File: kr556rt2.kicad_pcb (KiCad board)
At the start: 2 copper layers, 24.8 x 40.1 mm, 2 parts, among them U1 27C512, U2 КР556РТ2

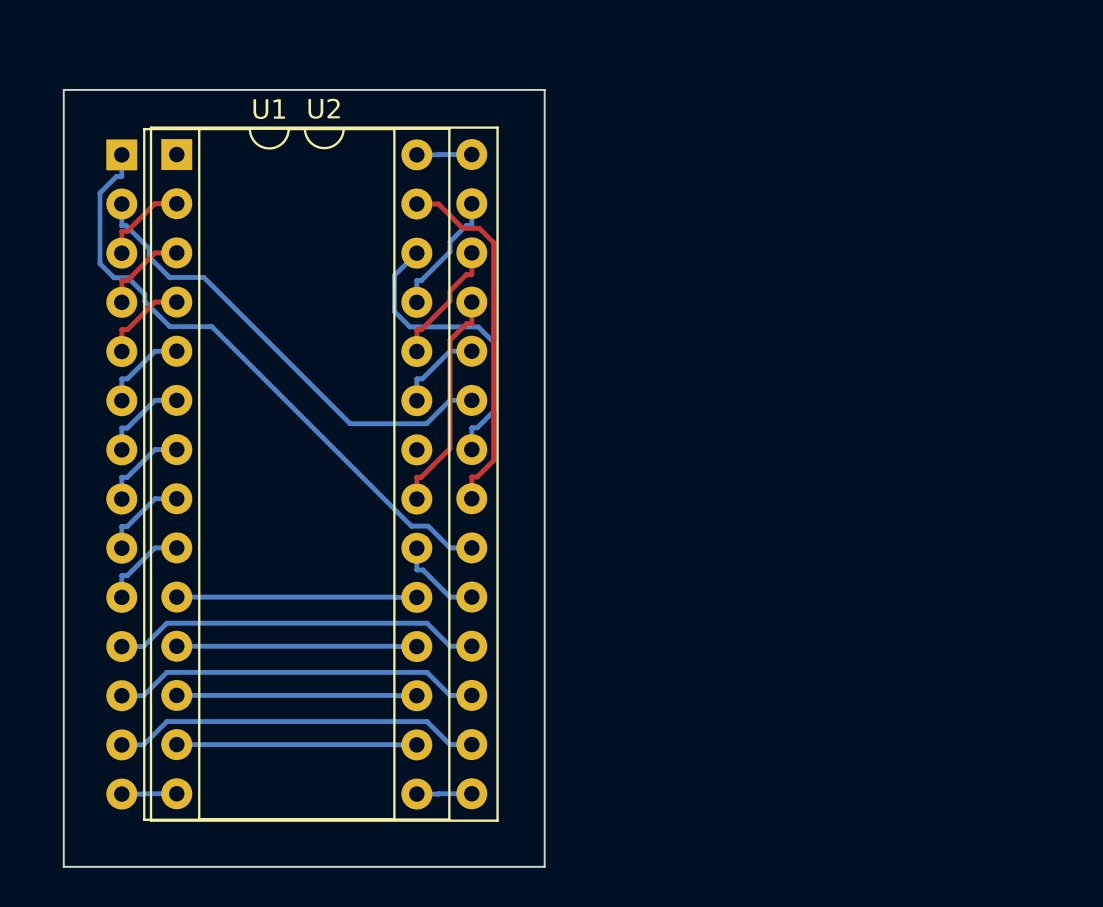
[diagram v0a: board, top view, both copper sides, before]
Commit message: Update kr556rt2.kicad_pcb
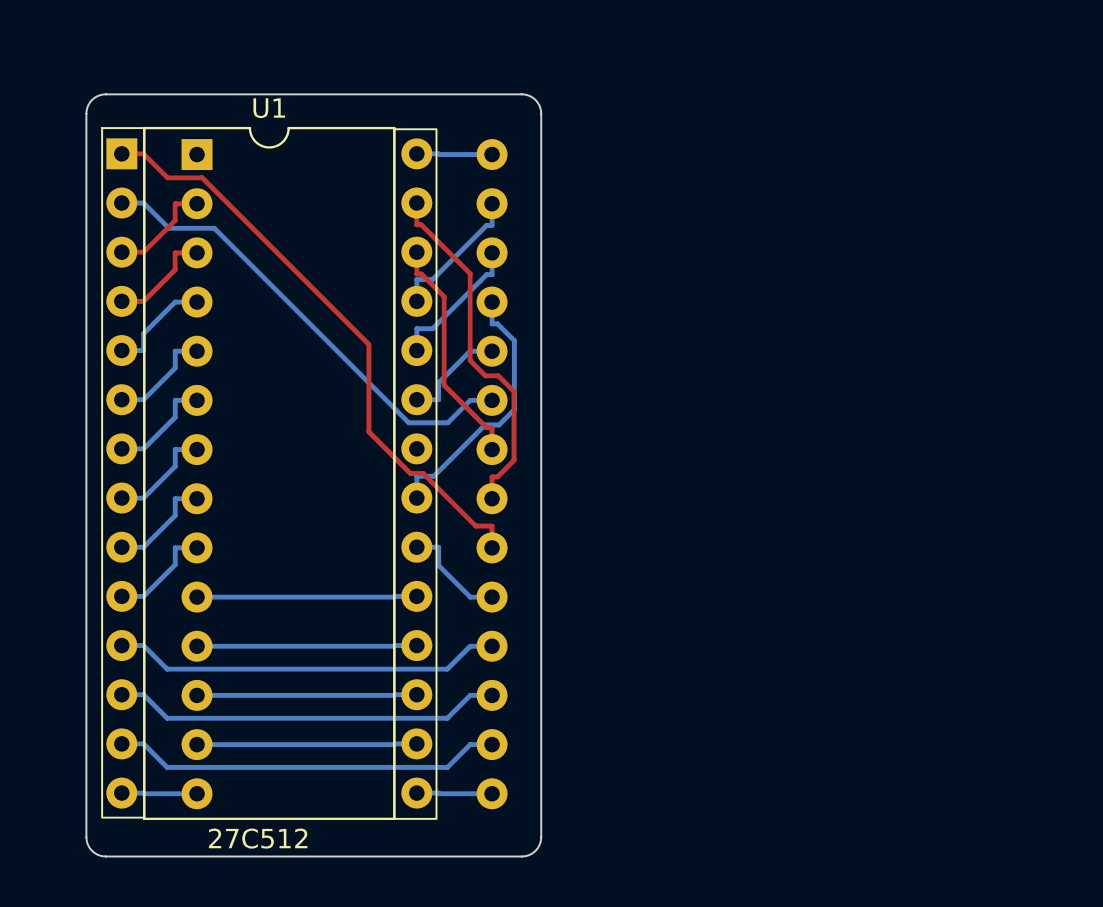
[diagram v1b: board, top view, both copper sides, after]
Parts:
- moved U2 1.05 mm to (66.7, 41.8)
- moved U1 0.05 mm to (62.8, 41.8)
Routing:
- net Net-(U1-A13): track 15.5 -> 12.1 mm
- net Net-(U1-A10): track 11.7 -> 13.8 mm
- net Net-(U1-VCC): track 2.85 -> 3.90 mm
- net Net-(U1-D3): track 2.85 -> 3.90 mm
- net Net-(U1-GND): track 2.85 -> 3.90 mm
- net Net-(U1-D0): track 19.1 -> 20.1 mm
- net Net-(U1-D2): track 19.1 -> 20.1 mm
- net Net-(U1-D1): track 19.1 -> 20.1 mm
- net Net-(U1-D7): track 12.4 -> 11.4 mm
- net Net-(U1-D5): track 12.4 -> 11.4 mm
- net Net-(U1-D6): track 12.4 -> 11.4 mm
- net Net-(U1-D4): track 12.4 -> 11.4 mm
- net Net-(U1-~{CE}): track 4.54 -> 5.51 mm
- net Net-(U1-A15): track 31.8 -> 30.9 mm
- net Net-(U1-A11): track 4.56 -> 5.43 mm
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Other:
- board size 24.8 x 40.1 mm -> 23.5 x 39.4 mm

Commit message: Update 22.07.2023 - Gerbers ver1
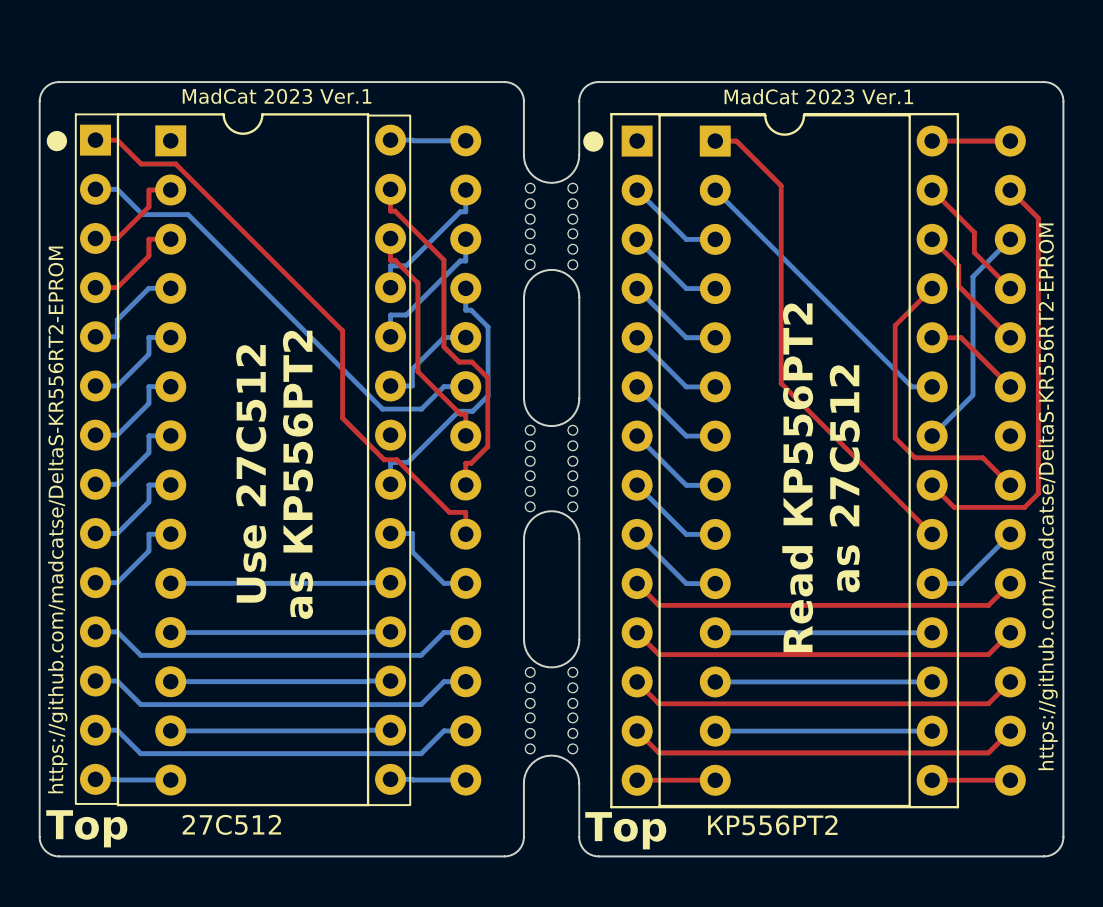
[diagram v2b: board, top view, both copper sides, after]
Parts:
- added U3: КР556РТ2, convertor_kr:DIP-28_W15.24mm_Socket, F.Cu at (89.4, 41.1)
- added U4: 27C512, convertor_kr:DIP-28_W15.24mm, F.Cu at (93.4, 41.1)
- added mouse-bite-2.54mm-slot_13: VAL**, convertor_kr:mouse-bite-2.54mm-slot, F.Cu at (85.0, 71.7)
- added mouse-bite-2.54mm-slot_13: VAL**, convertor_kr:mouse-bite-2.54mm-slot, F.Cu at (85.0, 69.4)
- added mouse-bite-2.54mm-slot_13: VAL**, convertor_kr:mouse-bite-2.54mm-slot, F.Cu at (85.0, 59.2)
- added mouse-bite-2.54mm-slot_13: VAL**, convertor_kr:mouse-bite-2.54mm-slot, F.Cu at (85.0, 46.7)
- added mouse-bite-2.54mm-slot_13: VAL**, convertor_kr:mouse-bite-2.54mm-slot, F.Cu at (85.0, 56.9)
- added mouse-bite-2.54mm-slot_13: VAL**, convertor_kr:mouse-bite-2.54mm-slot, F.Cu at (85.0, 44.4)
- U1: footprint Package_DIP:DIP-28_W15.24mm -> convertor_kr:DIP-28_W15.24mm
- U2: footprint Package_DIP:DIP-28_W15.24mm_Socket -> convertor_kr:DIP-28_W15.24mm_Socket
- moved U2 1.53 mm to (65.3, 41.1)
- moved U1 1.53 mm to (61.4, 41.1)
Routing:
- net Net-(U3-А16): track 0.00 -> 25.6 mm
- net Net-(U3-А15): track 0.00 -> 22.5 mm
- net Net-(U3-В8): track 0.00 -> 20.2 mm
- net Net-(U3-В7): track 0.00 -> 20.2 mm
- net Net-(U3-В6): track 0.00 -> 20.2 mm
- net Net-(U3-В5): track 0.00 -> 20.2 mm
- net Net-(U3-А11): track 0.00 -> 15.5 mm
- net Net-(U3-А13): track 0.00 -> 15.4 mm
- net Net-(U3-А14): track 0.00 -> 11.8 mm
- net Net-(U3-В3): track 0.00 -> 11.2 mm
- net Net-(U3-В2): track 0.00 -> 11.2 mm
- net Net-(U3-В1): track 0.00 -> 11.2 mm
- net Net-(U3-А9): track 0.00 -> 6.75 mm
- net Net-(U3-А10): track 0.00 -> 6.75 mm
- net Net-(U3-А2): track 0.00 -> 5.09 mm
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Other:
- board size 23.5 x 39.4 mm -> 52.9 x 40 mm
- board text added: "MadCat 2023 Ver.1"
- board text added: "Read КР556РТ2 as 27C512"
- board text added: "Top"
- board text added: "Use 27C512 as КР556РТ2"
- board text added: "https://github.com/madcatse/DeltaS-KR556RT2-EPROM"
- board text added: "https://t.me/zx_delta_s"
